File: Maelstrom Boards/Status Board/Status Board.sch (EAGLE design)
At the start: 14 parts, among them P1 39-30-04

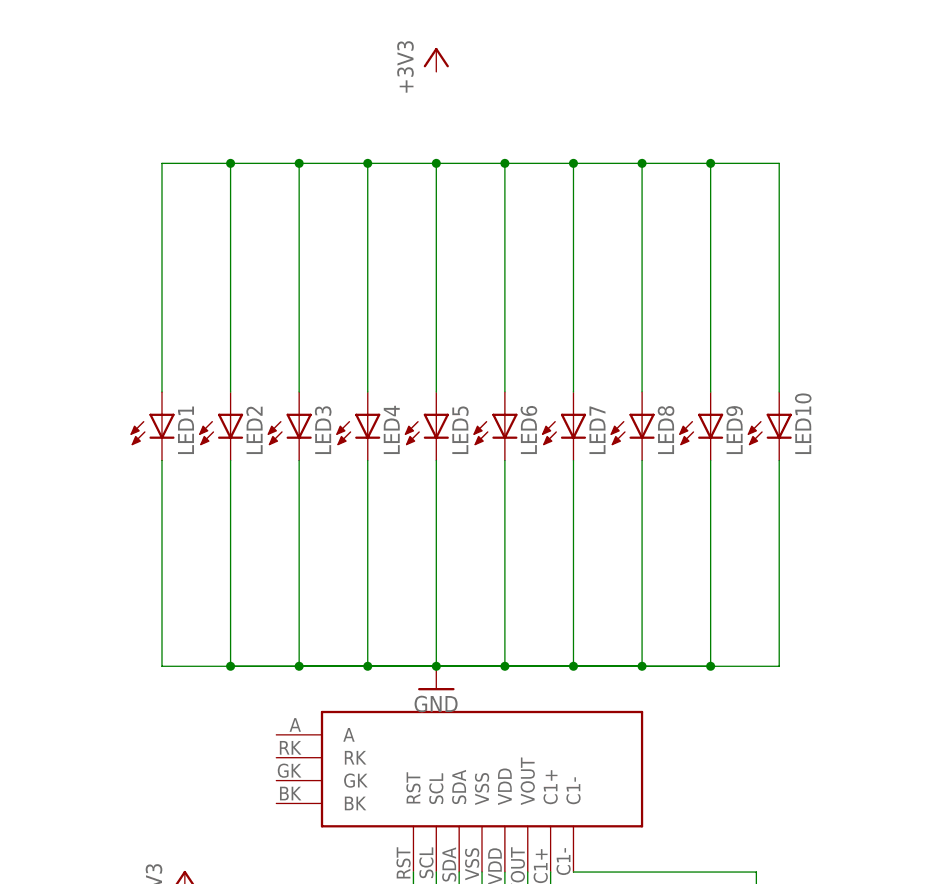
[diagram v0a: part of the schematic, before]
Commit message: Update Status Board
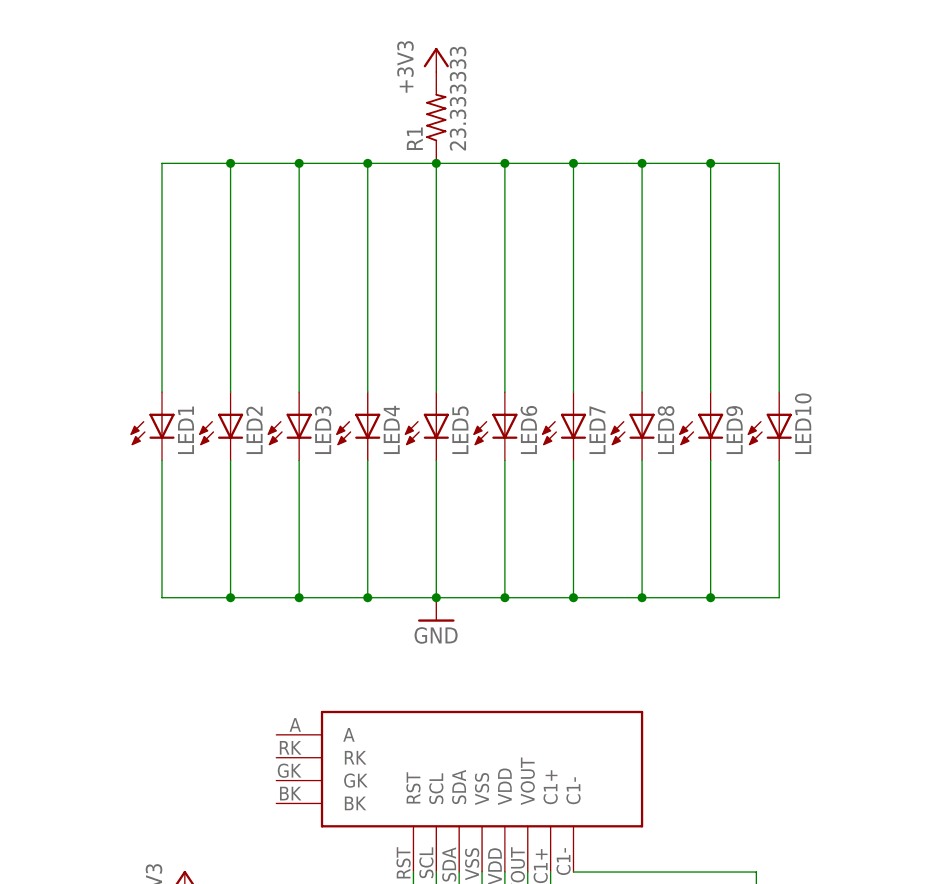
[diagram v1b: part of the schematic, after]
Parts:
- added R1: 23.333333, rcl:R-US_M3216
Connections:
- net +3V3: now also R1.2
- net N$4: now also R1.1
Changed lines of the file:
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@@
 <part name="LED10" library="led" library_urn="urn:adsk.eagle:library:259" deviceset="LED" device="CHIPLED_0603" package3d_urn="urn:adsk.eagle:package:15822/2"/>
 <part name="GND3" library="supply1" library_urn="urn:adsk.eagle:library:371" deviceset="GND" device=""/>
+<part name="R1" library="rcl" library_urn="urn:adsk.eagle:library:334" deviceset="R-US_" device="M3216" package3d_urn="urn:adsk.eagle:package:23563/1" value="23.333333"/>
 <part name="+3V3" library="supply1" library_urn="urn:adsk.eagle:library:371" deviceset="+3V3" device=""/>
 </parts>
@@
 <attribute name="VALUE" x="208.915" y="183.388" size="1.778" layer="96" rot="R90"/>
 </instance>
-<instance part="GND3" gate="1" x="165.1" y="157.48" smashed="yes">
-<attribute name="VALUE" x="162.56" y="154.94" size="1.778" layer="96"/>
+<instance part="GND3" gate="1" x="165.1" y="165.1" smashed="yes">
+<attribute name="VALUE" x="162.56" y="162.56" size="1.778" layer="96"/>
+</instance>
+<instance part="R1" gate="G$1" x="165.1" y="220.98" smashed="yes" rot="R90">
+<attribute name="NAME" x="163.6014" y="217.17" size="1.778" layer="95" rot="R90"/>
+<attribute name="VALUE" x="168.402" y="217.17" size="1.778" layer="96" rot="R90"/>
 </instance>
 <instance part="+3V3" gate="G$1" x="165.1" y="228.6" smashed="yes">
@@
 <junction x="162.56" y="134.62"/>
 </segment>
+<segment>
+<pinref part="+3V3" gate="G$1" pin="+3V3"/>
+<pinref part="R1" gate="G$1" pin="2"/>
+</segment>
 </net>
 <net name="GND" class="0">
@@
 <pinref part="LED5" gate="G$1" pin="C"/>
 <pinref part="GND3" gate="1" pin="GND"/>
-<wire x1="165.1" y1="182.88" x2="165.1" y2="160.02" width="0.1524" layer="91"/>
+<wire x1="165.1" y1="182.88" x2="165.1" y2="167.64" width="0.1524" layer="91"/>
 <pinref part="LED4" gate="G$1" pin="C"/>
-<wire x1="157.48" y1="182.88" x2="157.48" y2="160.02" width="0.1524" layer="91"/>
-<wire x1="157.48" y1="160.02" x2="165.1" y2="160.02" width="0.1524" layer="91"/>
-<junction x="165.1" y="160.02"/>
+<wire x1="157.48" y1="182.88" x2="157.48" y2="167.64" width="0.1524" layer="91"/>
+<junction x="165.1" y="167.64"/>
 <pinref part="LED3" gate="G$1" pin="C"/>
-<wire x1="149.86" y1="182.88" x2="149.86" y2="160.02" width="0.1524" layer="91"/>
-<wire x1="149.86" y1="160.02" x2="157.48" y2="160.02" width="0.1524" layer="91"/>
+<wire x1="149.86" y1="182.88" x2="149.86" y2="167.64" width="0.1524" layer="91"/>
 <pinref part="LED2" gate="G$1" pin="C"/>
-<wire x1="157.48" y1="160.02" x2="165.1" y2="160.02" width="0.1524" layer="91"/>
-<wire x1="142.24" y1="182.88" x2="142.24" y2="160.02" width="0.1524" layer="91"/>
-<wire x1="142.24" y1="160.02" x2="149.86" y2="160.02" width="0.1524" layer="91"/>
+<wire x1="142.24" y1="182.88" x2="142.24" y2="167.64" width="0.1524" layer="91"/>
 <pinref part="LED1" gate="G$1" pin="C"/>
-<wire x1="149.86" y1="160.02" x2="157.48" y2="160.02" width="0.1524" layer="91"/>
-<wire x1="157.48" y1="160.02" x2="165.1" y2="160.02" width="0.1524" layer="91"/>
-<wire x1="134.62" y1="182.88" x2="134.62" y2="160.02" width="0.1524" layer="91"/>
-<wire x1="134.62" y1="160.02" x2="142.24" y2="160.02" width="0.1524" layer="91"/>
+<wire x1="134.62" y1="182.88" x2="134.62" y2="167.64" width="0.1524" layer="91"/>
+<wire x1="134.62" y1="167.64" x2="142.24" y2="167.64" width="0.1524" layer="91"/>
 <pinref part="LED6" gate="G$1" pin="C"/>
-<wire x1="142.24" y1="160.02" x2="149.86" y2="160.02" width="0.1524" layer="91"/>
-<wire x1="149.86" y1="160.02" x2="157.48" y2="160.02" width="0.1524" layer="91"/>
-<wire x1="157.48" y1="160.02" x2="165.1" y2="160.02" width="0.1524" layer="91"/>
-<wire x1="172.72" y1="182.88" x2="172.72" y2="160.02" width="0.1524" layer="91"/>
-<wire x1="172.72" y1="160.02" x2="165.1" y2="160.02" width="0.1524" layer="91"/>
+<wire x1="142.24" y1="167.64" x2="149.86" y2="167.64" width="0.1524" layer="91"/>
+<wire x1="149.86" y1="167.64" x2="157.48" y2="167.64" width="0.1524" layer="91"/>
+<wire x1="157.48" y1="167.64" x2="165.1" y2="167.64" width="0.1524" layer="91"/>
+<wire x1="172.72" y1="182.88" x2="172.72" y2="167.64" width="0.1524" layer="91"/>
 <pinref part="LED7" gate="G$1" pin="C"/>
-<wire x1="180.34" y1="182.88" x2="180.34" y2="160.02" width="0.1524" layer="91"/>
-<wire x1="180.34" y1="160.02" x2="172.72" y2="160.02" width="0.1524" layer="91"/>
+<wire x1="180.34" y1="182.88" x2="180.34" y2="167.64" width="0.1524" layer="91"/>
 <pinref part="LED8" gate="G$1" pin="C"/>
-<wire x1="172.72" y1="160.02" x2="165.1" y2="160.02" width="0.1524" layer="91"/>
-<wire x1="187.96" y1="182.88" x2="187.96" y2="160.02" width="0.1524" layer="91"/>
-<wire x1="187.96" y1="160.02" x2="180.34" y2="160.02" width="0.1524" layer="91"/>
+<wire x1="187.96" y1="182.88" x2="187.96" y2="167.64" width="0.1524" layer="91"/>
 <pinref part="LED9" gate="G$1" pin="C"/>
-<wire x1="180.34" y1="160.02" x2="172.72" y2="160.02" width="0.1524" layer="91"/>
-<wire x1="172.72" y1="160.02" x2="165.1" y2="160.02" width="0.1524" layer="91"/>
-<wire x1="195.58" y1="182.88" x2="195.58" y2="160.02" width="0.1524" layer="91"/>
-<wire x1="195.58" y1="160.02" x2="187.96" y2="160.02" width="0.1524" layer="91"/>
+<wire x1="195.58" y1="182.88" x2="195.58" y2="167.64" width="0.1524" layer="91"/>
 <pinref part="LED10" gate="G$1" pin="C"/>
-<wire x1="187.96" y1="160.02" x2="180.34" y2="160.02" width="0.1524" layer="91"/>
-<wire x1="180.34" y1="160.02" x2="172.72" y2="160.02" width="0.1524" layer="91"/>
-<wire x1="172.72" y1="160.02" x2="165.1" y2="160.02" width="0.1524" layer="91"/>
-<wire x1="203.2" y1="182.88" x2="203.2" y2="160.02" width="0.1524" layer="91"/>
-<wire x1="203.2" y1="160.02" x2="195.58" y2="160.02" width="0.1524" layer="91"/>
-<junction x="195.58" y="160.02"/>
-<wire x1="195.58" y1="160.02" x2="187.96" y2="160.02" width="0.1524" layer="91"/>
-<junction x="187.96" y="160.02"/>
-<wire x1="187.96" y1="160.02" x2="180.34" y2="160.02" width="0.1524" layer="91"/>
-<junction x="180.34" y="160.02"/>
-<wire x1="180.34" y1="160.02" x2="172.72" y2="160.02" width="0.1524" layer="91"/>
-<junction x="172.72" y="160.02"/>
-<wire x1="172.72" y1="160.02" x2="165.1" y2="160.02" width="0.1524" layer="91"/>
-<junction x="157.48" y="160.02"/>
-<junction x="149.86" y="160.02"/>
-<junction x="142.24" y="160.02"/>
+<wire x1="203.2" y1="182.88" x2="203.2" y2="167.64" width="0.1524" layer="91"/>
+<wire x1="203.2" y1="167.64" x2="195.58" y2="167.64" width="0.1524" layer="91"/>
+<junction x="195.58" y="167.64"/>
+<wire x1="195.58" y1="167.64" x2="187.96" y2="167.64" width="0.1524" layer="91"/>
+<junction x="187.96" y="167.64"/>
+<wire x1="187.96" y1="167.64" x2="180.34" y2="167.64" width="0.1524" layer="91"/>
+<junction x="180.34" y="167.64"/>
+<wire x1="180.34" y1="167.64" x2="172.72" y2="167.64" width="0.1524" layer="91"/>
+<junction x="172.72" y="167.64"/>
+<wire x1="172.72" y1="167.64" x2="165.1" y2="167.64" width="0.1524" layer="91"/>
+<junction x="157.48" y="167.64"/>
+<junction x="149.86" y="167.64"/>
+<junction x="142.24" y="167.64"/>
 </segment>
 </net>
@@
 <junction x="187.96" y="215.9"/>
 <junction x="195.58" y="215.9"/>
+<pinref part="R1" gate="G$1" pin="1"/>
 </segment>
 </net>

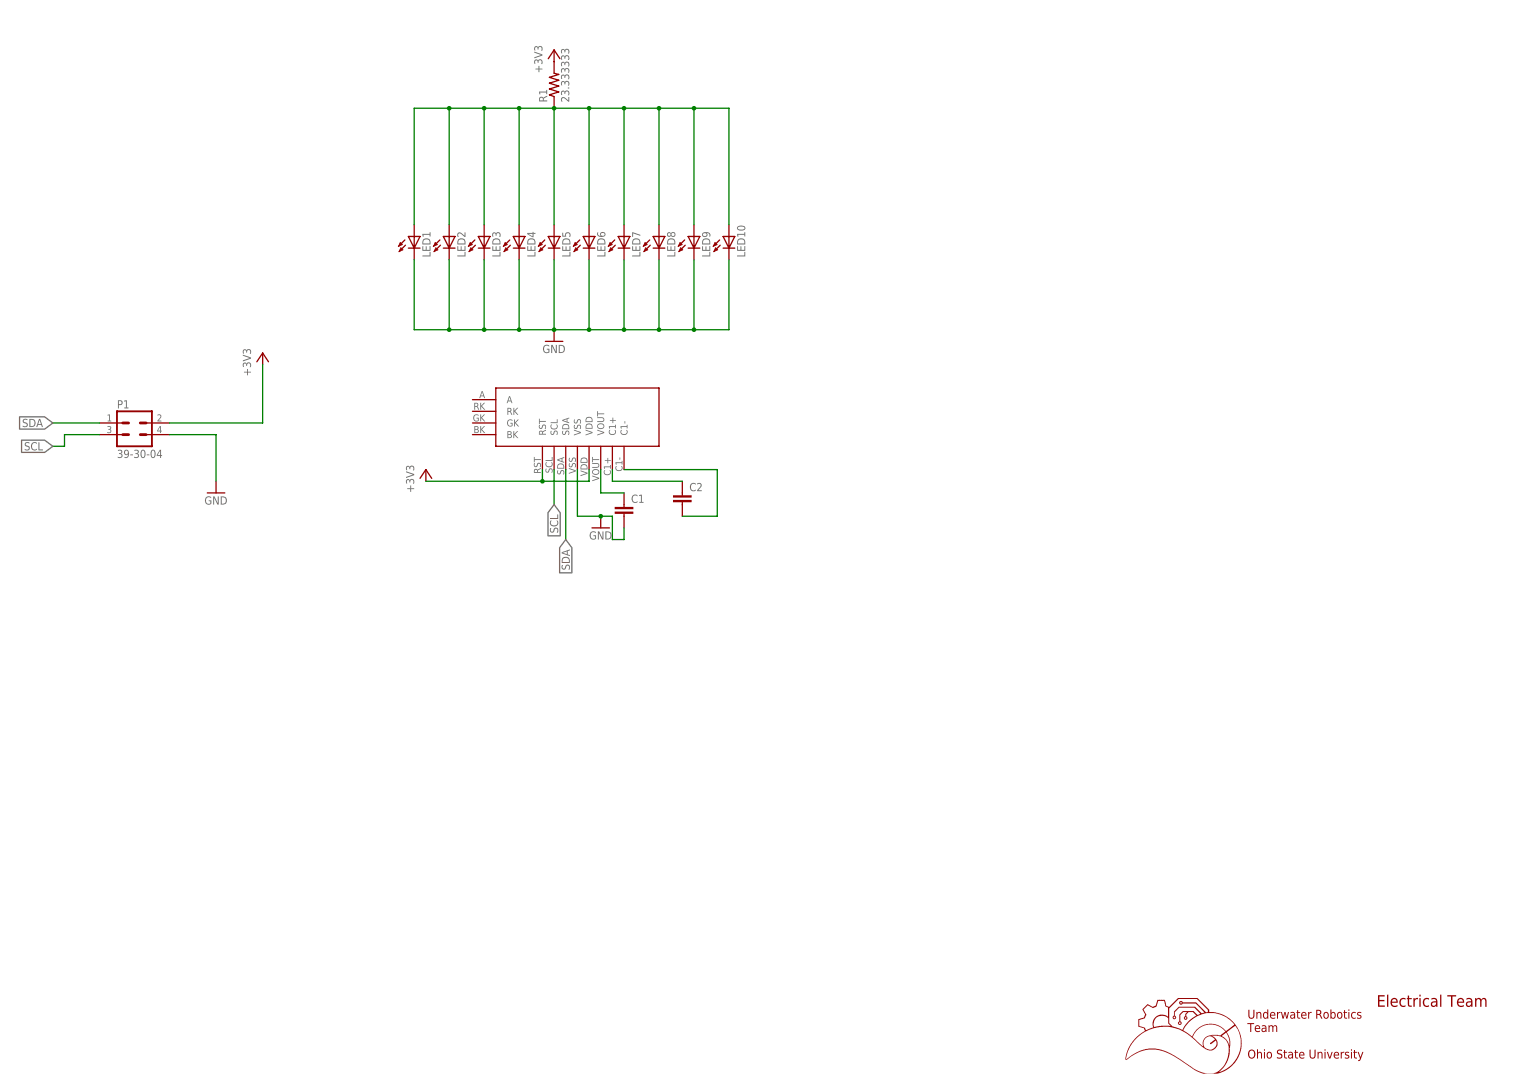
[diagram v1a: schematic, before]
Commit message: Finished status board schematic
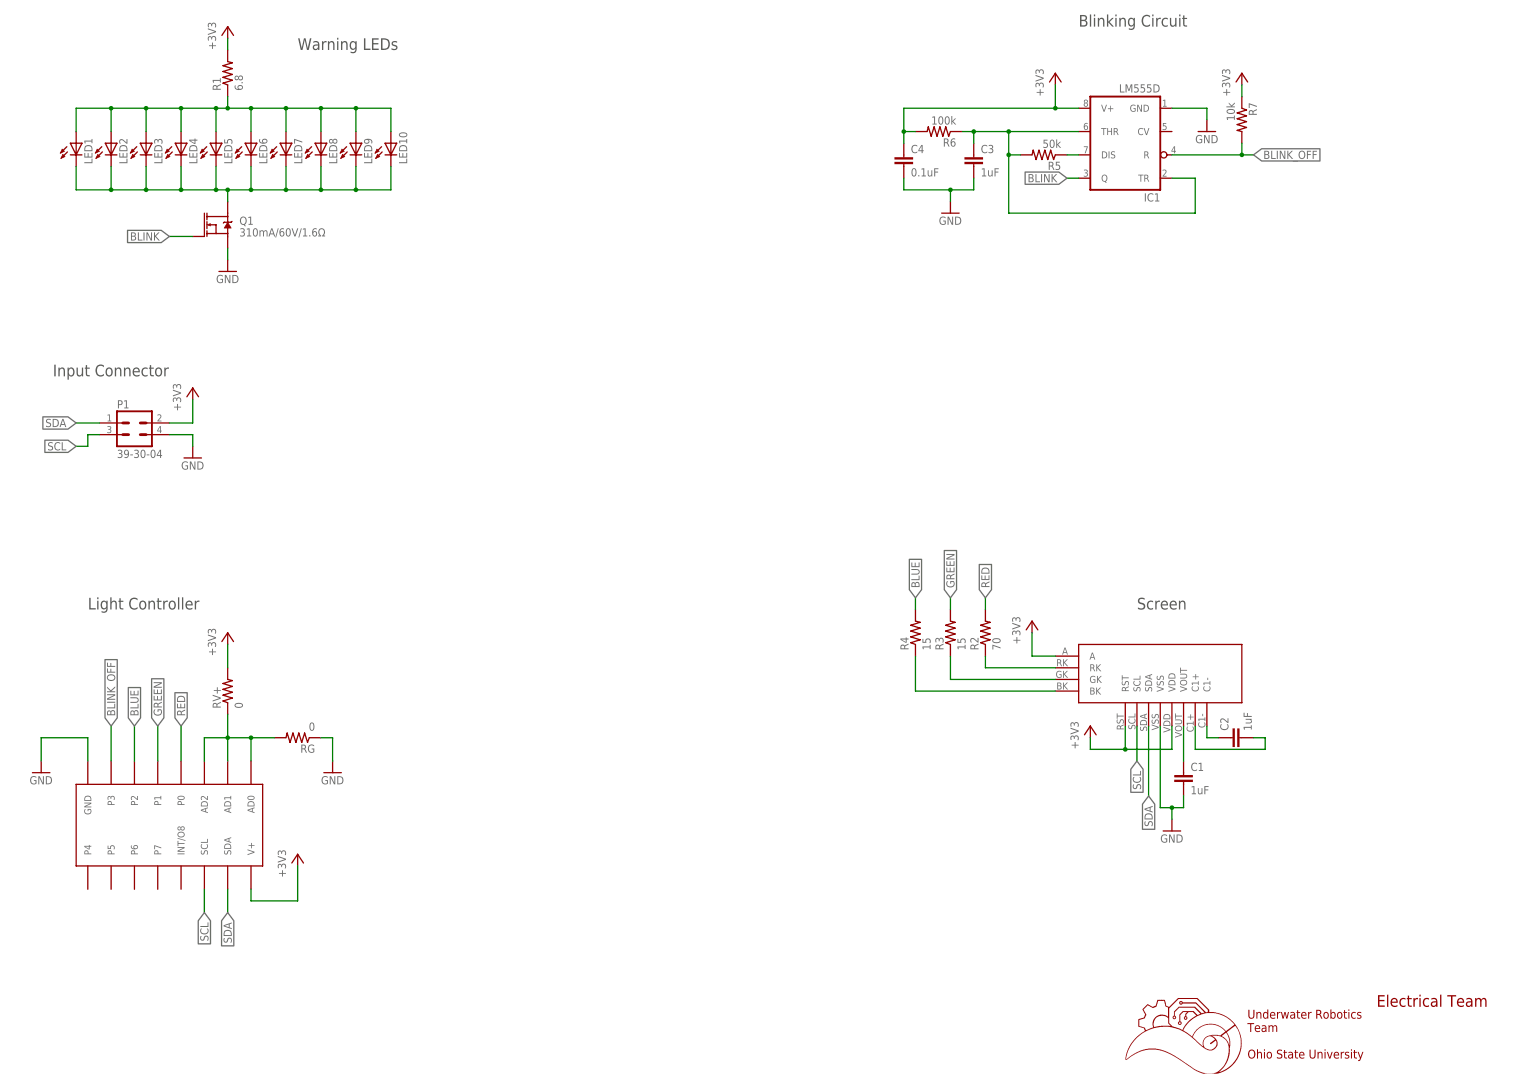
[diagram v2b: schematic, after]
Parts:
- added C3: 1uF, rcl:C-EUC0603
- added C4: 0.1uF, rcl:C-EUC0603
- added IC1: LM555D, linear:LM555D
- added Q1: 310mA/60V/1.6Ω, SparkFun-DiscreteSemi:MOSFET-NCH-2N7002PW
- added R2: 70, rcl:R-US_R0603
- added R3, R4: 15, rcl:R-US_R0603
- added R5: 50k, rcl:R-US_R0603
- added R6: 100k, rcl:R-US_R0603
- added R7: 10k, rcl:R-US_R0603
- added RG, RV+: 0, rcl:R-US_R0603
- added U$2: MAX7315, MAX7315:MAX7315
- C1, C2: value (none) -> 1uF
- R1: value 23.333333 -> 6.8; device rcl:R-US_M3216 -> rcl:R-US_R0603
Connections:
- new net BLINK: IC1.Q, Q1.G
- new net BLINK_OFF: IC1.R, R7.2, U$2.P3
- new net BLUE: R4.2, U$2.P2
- new net GREEN: R3.2, U$2.P1
- new net N$10: C3.1, IC1.THR, IC1.TR, R5.2, R6.1
- new net N$20: LED1.C, LED10.C, LED2.C, LED3.C, LED4.C, LED5.C, LED6.C, LED7.C, LED8.C, LED9.C, Q1.D
- new net N$4: C2.2, U$1.C1+
- new net N$5: R3.1, U$1.GK
- new net N$6: RG.2, RV+.1, U$2.AD0, U$2.AD1, U$2.AD2
- new net N$7: R2.1, U$1.RK
- new net N$9: IC1.DIS, R5.1
- new net RED: R2.2, U$2.P0
- net +3V3: now also C4.1, IC1.V+, R6.2, R7.1, RV+.2, U$1.A, U$2.V+
- net GND: now also C3.2, C4.2, IC1.GND, Q1.S, RG.1, U$2.GND; no longer LED1.C, LED10.C, LED2.C, LED3.C, LED4.C, LED5.C, LED6.C, LED7.C, LED8.C, LED9.C
- net N$1: now also R4.1, U$1.BK; no longer C2.1, U$1.C1+
- net N$2: now also C2.1; no longer C2.2
- net SCL: now also U$2.SCL
- net SDA: now also U$2.SDA
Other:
- note added: "Blinking Circuit"
- note added: "Input Connector"
- note added: "Light Controller"
- note added: "Screen"
- note added: "Warning LEDs"
- moved on the sheet: C1, C2, LED1, LED10, LED2, LED3, LED4, LED5, LED6, LED7, LED8, LED9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
